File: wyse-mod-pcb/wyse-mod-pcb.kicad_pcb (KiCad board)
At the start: 2 copper layers, 27.9 x 33.5 mm, 12 parts, among them J1 RJ9, J2 Handwire, SW1 Reset Switch, U1 ProMicro

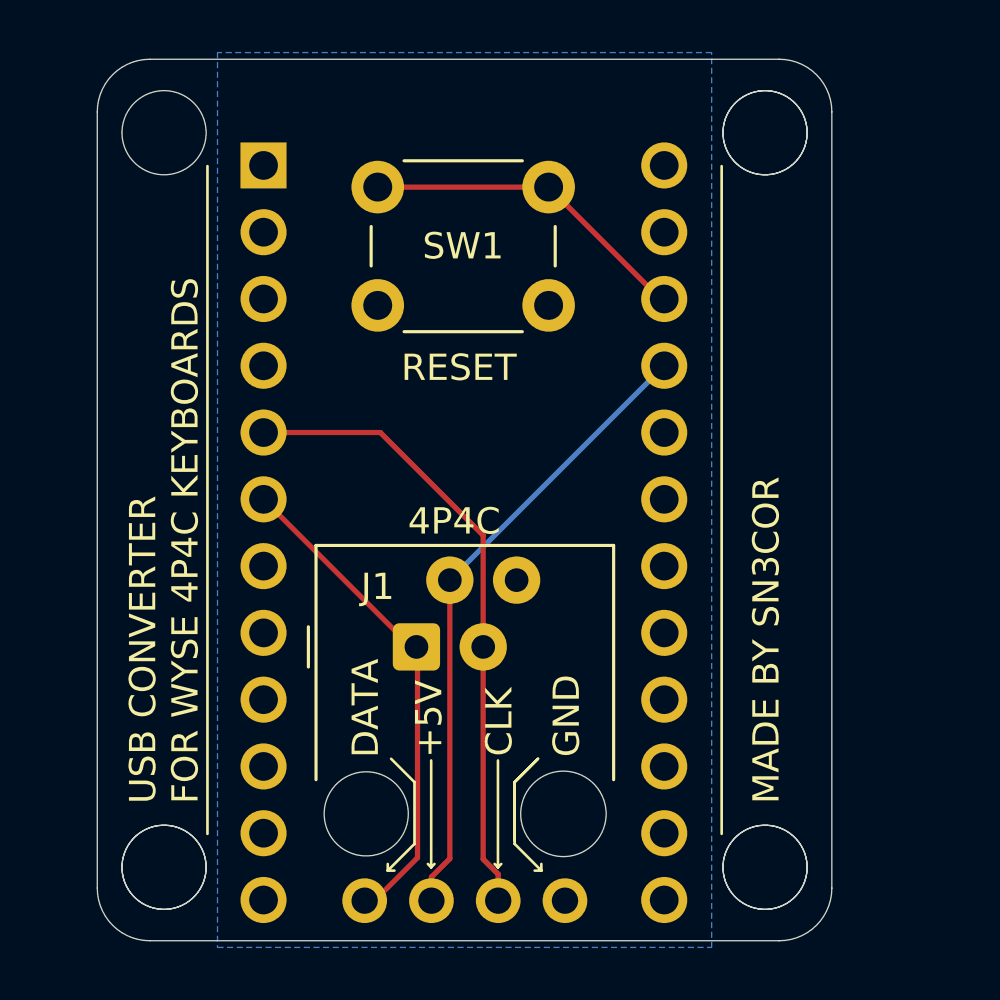
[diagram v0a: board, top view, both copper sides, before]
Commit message: Added assets
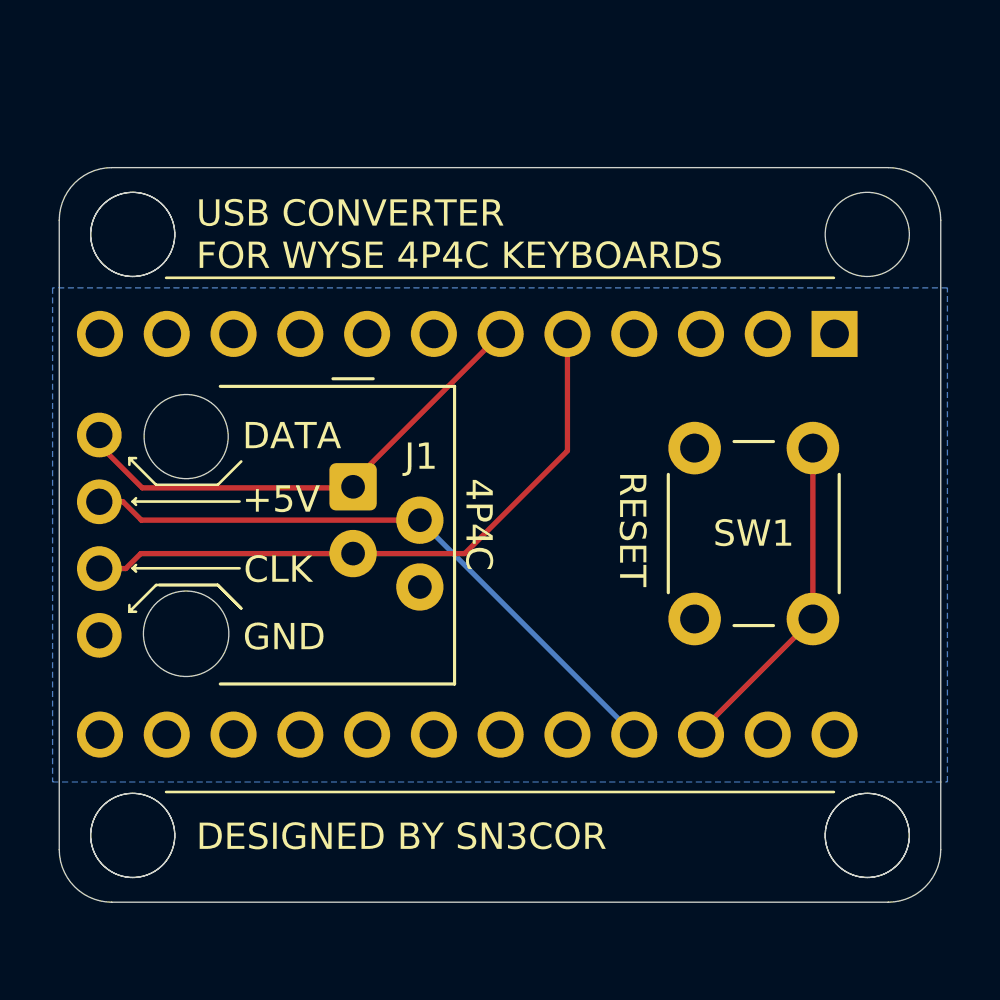
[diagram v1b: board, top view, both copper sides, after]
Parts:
- moved REF** 27.0 mm to (174.1, 90.2), turned to -90 degrees
- moved ? 27.0 mm to (174.1, 113.1), turned to -90 degrees
- moved REF** 27.0 mm to (174.1, 113.1), turned to -90 degrees
- moved ? 24.1 mm to (146.1, 90.2), turned to -90 degrees
- moved REF** 24.1 mm to (146.1, 90.2), turned to -90 degrees
- moved ? 24.1 mm to (146.1, 113.1), turned to -90 degrees
- moved REF** 24.1 mm to (146.1, 113.1), turned to -90 degrees
- moved J2 20.4 mm to (144.9, 97.9), turned to 0 degrees
- moved SW1 19.3 mm to (172.0, 98.4), turned to -90 degrees
- moved G*** 18.4 mm to (164.8, 113.2), turned to 180 degrees
- moved J1 6.55 mm to (154.5, 99.8), turned to -90 degrees
- moved U1 0.14 mm to (158.9, 101.6), turned to 180 degrees
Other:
- board size 27.9 x 33.5 mm -> 33.5 x 27.9 mm
- board text added: "DESIGNED BY SN3COR"
- board text added: "FLIP THE PRO MICRO SO THE USB IS FACING THE PCB"
- board text removed: "FLIP THE PRO MICRO SO THAT THE USB IS FACING THE PCB"
- board text removed: "MADE BY SN3COR"
